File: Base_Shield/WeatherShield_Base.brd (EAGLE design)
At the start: 58.4 x 67.3 mm, 73 parts, among them Q1 BSS138, Q2 BSS138, U1 DS3231SN, U2 LT3652, U3 TMP100MDBVREP, U4 ADS1015IDGST

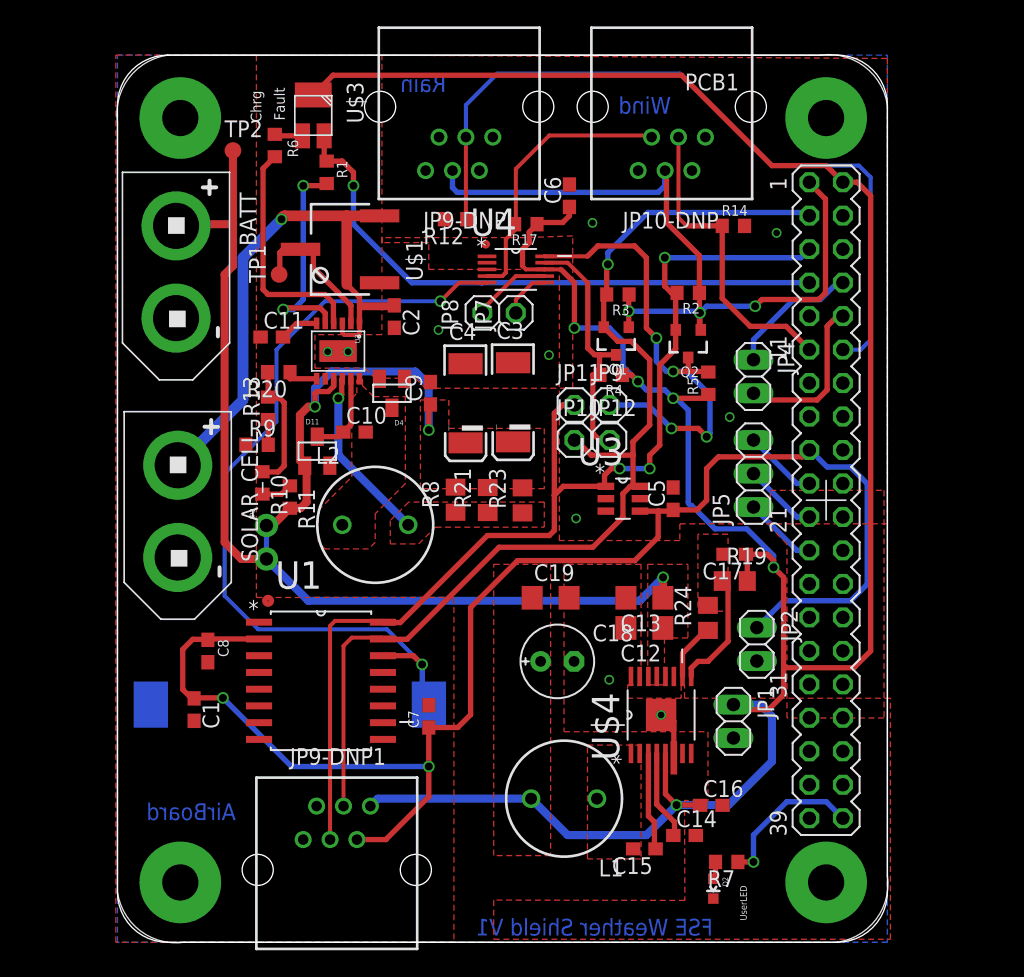
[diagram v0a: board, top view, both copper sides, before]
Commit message: WeatherShield_v1
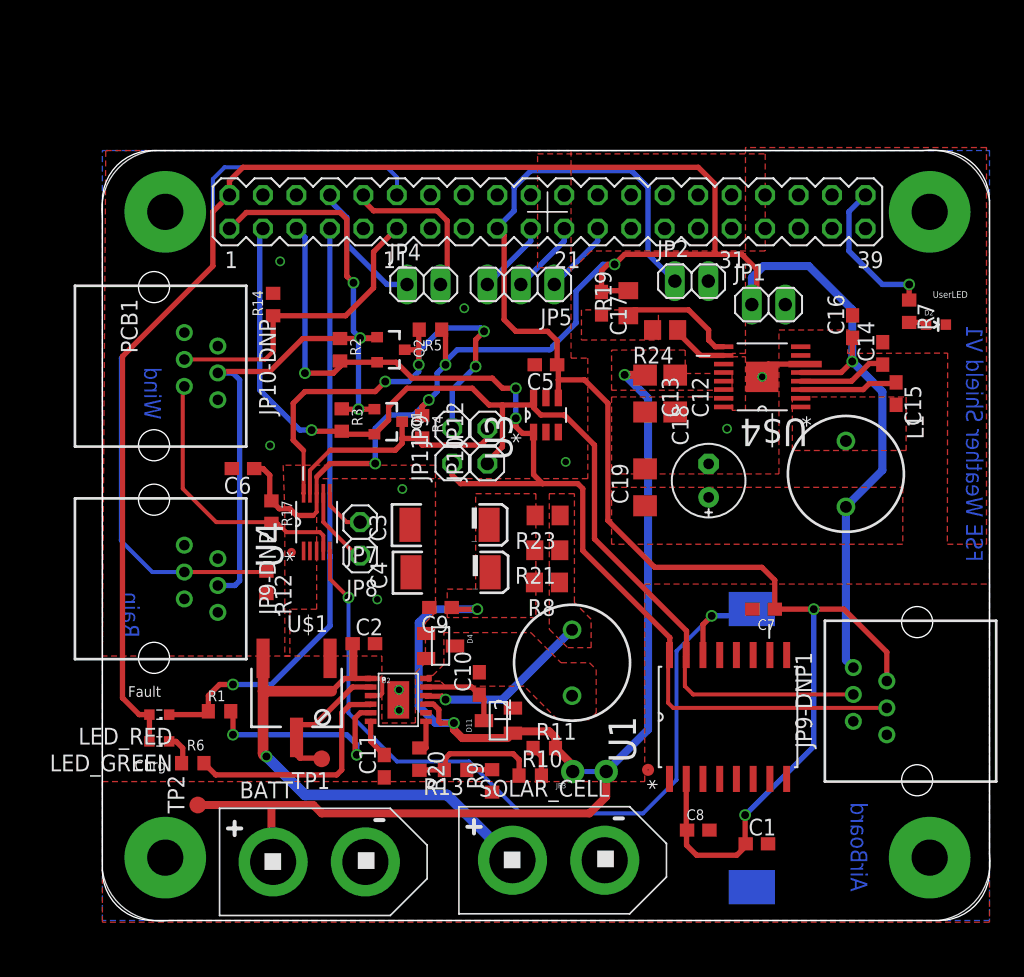
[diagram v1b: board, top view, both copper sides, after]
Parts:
- removed U$3: VLMV3100, FSEWeatherShield:VLMV3100
- added LED_GREEN, LED_RED: (no value), led:SML0603
- moved PCB1 65.7 mm to (0.00, 2.67), turned to 0 degrees
- moved JP9-DNP1 57.6 mm to (67.8, 13.2), turned to 90 degrees
- moved JP10-DNP 55.0 mm to (-2.08, 50.8), turned to 270 degrees
- moved JP9-DNP 50.2 mm to (-2.08, 34.7), turned to 270 degrees
- moved TP2 49.7 mm to (7.24, 11.4), turned to 90 degrees
- moved BATT 48.8 mm to (13.0, 7.11), turned to 0 degrees
- moved R6 47.3 mm to (6.86, 14.6), turned to 0 degrees
- moved D2 46.0 mm to (63.2, 47.9), turned to 270 degrees
- moved R7 44.0 mm to (61.2, 48.9), turned to 270 degrees
- moved C1 43.9 mm to (49.7, 8.48), turned to 0 degrees
- moved R1 41.7 mm to (8.89, 18.5), turned to 0 degrees
- moved C8 39.6 mm to (45.2, 9.53), turned to 0 degrees
- moved C14 39.5 mm to (59.2, 45.7), turned to 90 degrees
- moved C15 39.5 mm to (60.2, 42.6), turned to 270 degrees
- moved SOLAR_CELL 39.3 mm to (31.1, 7.24), turned to 0 degrees
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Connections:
- net 5V: now also LED_GREEN.A, LED_RED.A; no longer U$3.C
- net FAULT_PIN: now also LED_RED.C; no longer U$3.A_RED
- net N$4: now also LED_GREEN.C; no longer U$3.A_GREEN
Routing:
- net 5V: track 202.2 -> 204.2 mm
- net FAULT_PIN: track 45.1 -> 46.2 mm
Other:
- board size 58.4 x 67.3 mm -> 67.3 x 58.4 mm
